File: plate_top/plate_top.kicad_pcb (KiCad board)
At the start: 2 copper layers, 179.7 x 122.7 mm, 44 parts, among them SW1 SW_Push, SW10 SW_Push, SW11 SW_Push, SW12 SW_Push, SW13 SW_Push, SW14 SW_Push, SW15 SW_Push, SW16 SW_Push, SW17 SW_Push, SW18 SW_Push, SW19 SW_Push, SW2 SW_Push, SW20 SW_Push, SW21 SW_Push, SW22 SW_Push, SW23 SW_Push, SW24 SW_Push, SW25 SW_Push, SW26 SW_Push, SW27 SW_Push, SW28 SW_Push, SW29 SW_Push, SW3 SW_Push, SW30 SW_Push, SW31 SW_Push, SW32 SW_Push, SW4 SW_Push, SW5 SW_Push, SW6 SW_Push, SW7 SW_Push, SW8 SW_Push, SW9 SW_Push

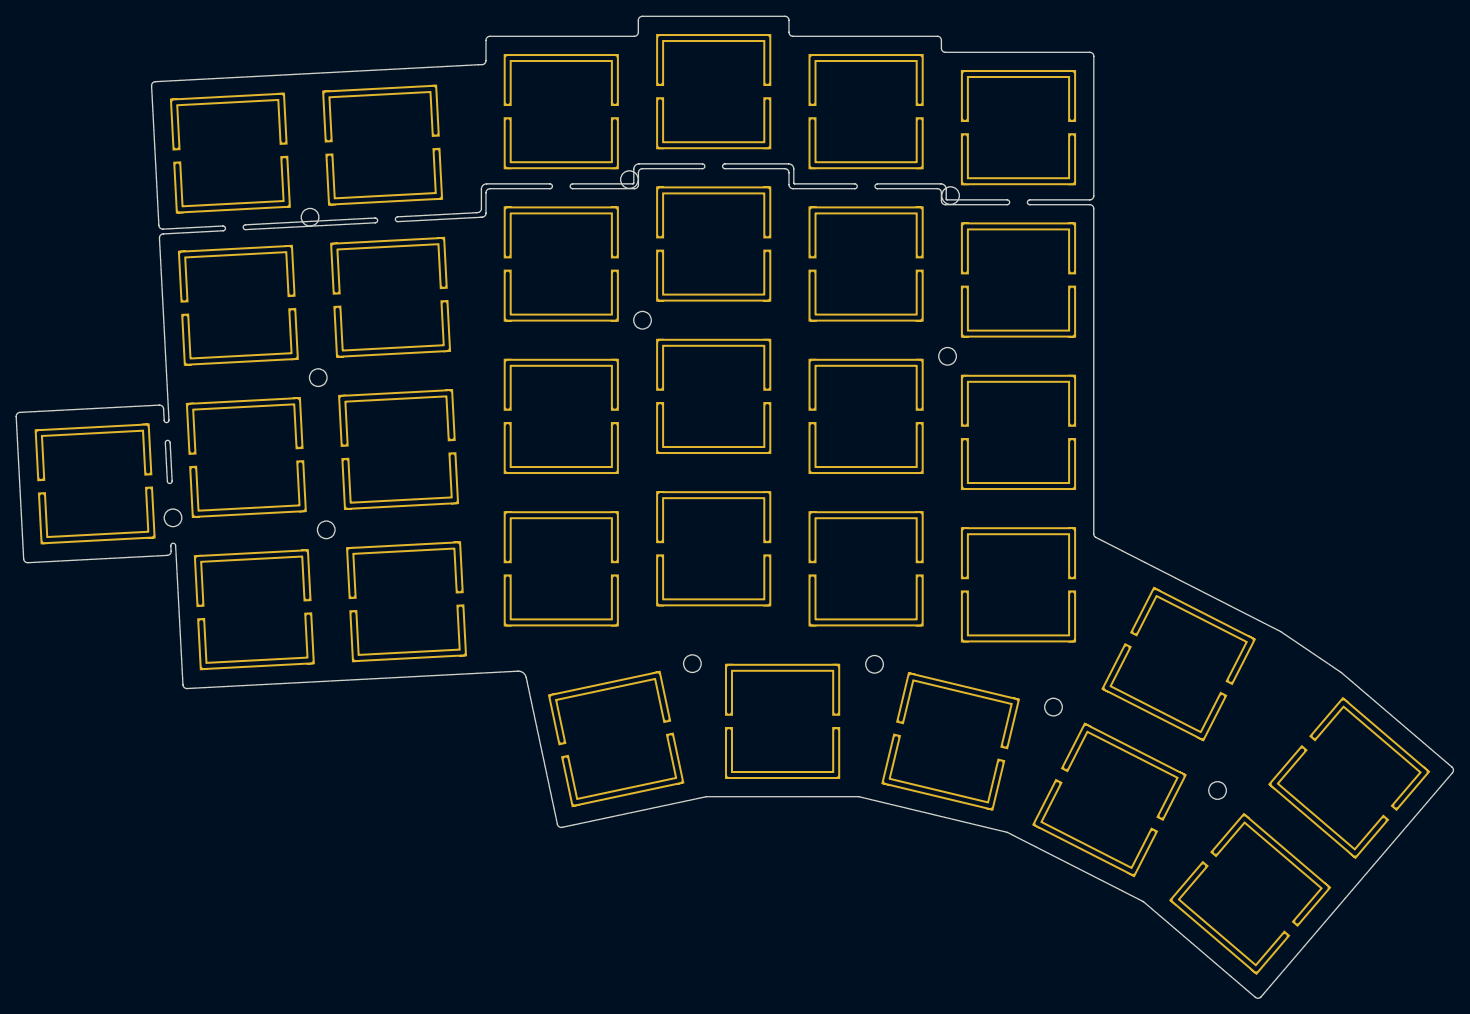
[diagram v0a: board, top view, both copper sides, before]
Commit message: Final changes of palm release.
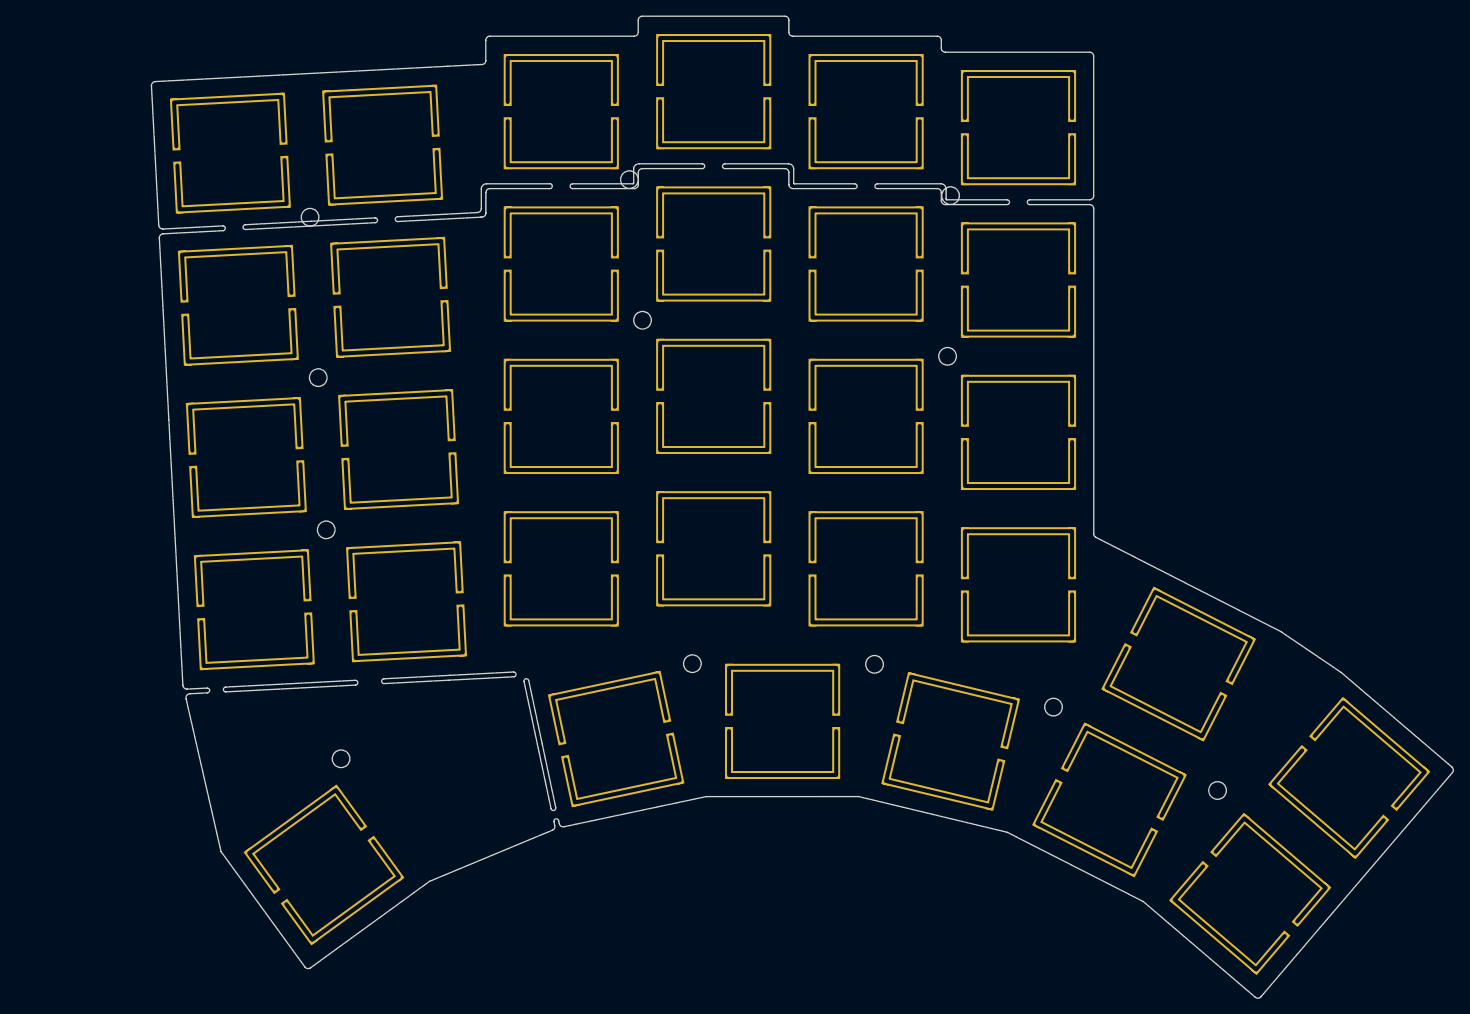
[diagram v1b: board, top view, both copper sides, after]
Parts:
- moved SW27 55.6 mm to (90.0, 136.1), turned to 216 degrees
- moved HM5 36.7 mm to (92.1, 122.8)
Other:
- board size 179.7 x 122.7 mm -> 162.7 x 122.7 mm
